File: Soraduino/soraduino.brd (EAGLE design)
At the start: 87.3 x 81.3 mm, 23 parts, among them IC1 ATMEGA168-AU, IC2 317EMP, IC3 317EMP

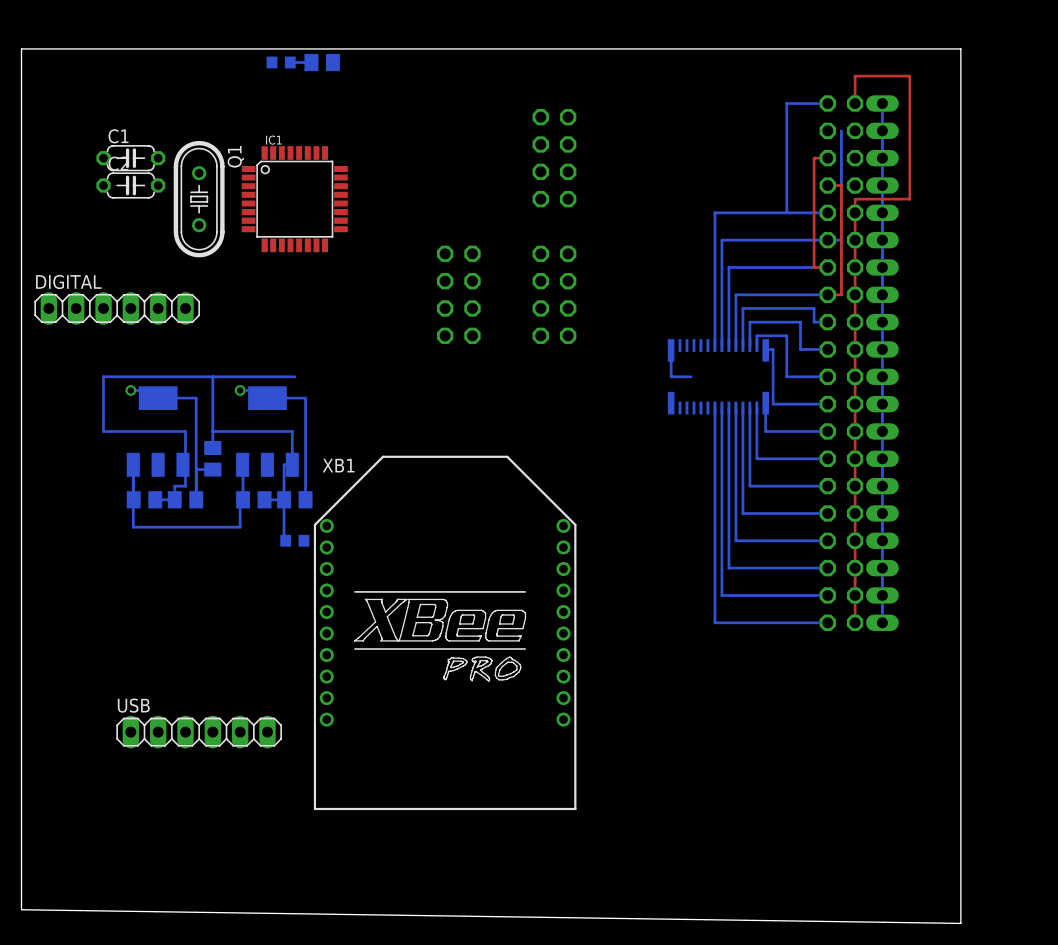
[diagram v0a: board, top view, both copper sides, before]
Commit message: 回路をとりあえず完成
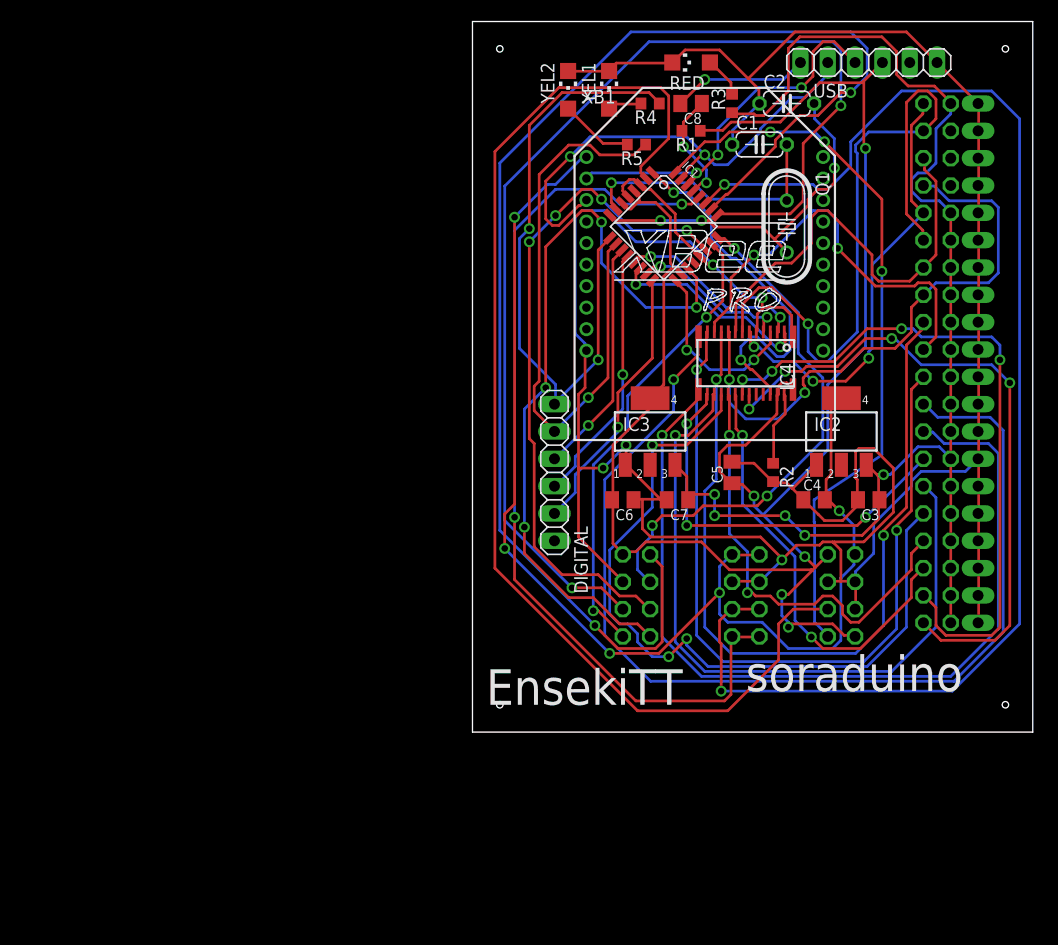
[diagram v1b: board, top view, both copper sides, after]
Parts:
- added R3, R4, R5: 1k, rcl:R0603
- added RED, YEL1, YEL2: (no value), led:CHIPLED_1206
- moved USB 88.0 mm to (91.4, 81.3)
- moved C2 61.4 mm to (83.8, 77.5)
- moved C1 58.4 mm to (81.3, 73.7)
- moved C3 57.1 mm to (91.4, 40.6), flipped to the top
- moved Q1 54.7 mm to (83.8, 66.0)
- moved IC2 53.3 mm to (88.9, 47.0), flipped to the top
- moved C7 49.5 mm to (73.7, 40.6), flipped to the top
- moved C5 48.3 mm to (78.7, 43.2), flipped to the top
- moved C4 48.3 mm to (86.4, 40.6), flipped to the top, turned to 0 degrees
- moved IC3 45.7 mm to (71.1, 47.0), flipped to the top
- moved GPS-SUP 45.2 mm to (88.9, 31.8)
- moved R2 44.9 mm to (82.5, 43.2), flipped to the top, turned to 270 degrees
- moved DIGITAL 43.4 mm to (62.2, 43.2), turned to 270 degrees
- moved XB1 41.9 mm to (76.2, 63.5)
- moved JAIRO-ANA 41.3 mm to (69.8, 31.8)
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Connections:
- new net N$10: R3.2, RED.A
- new net N$46: R4.2, YEL1.A
- new net N$48: R5.2, YEL2.A
- net GND: now also RED.C, YEL1.C, YEL2.C
- net N$39: now also R4.1
- net N$40: now also R5.1
- net VCC: now also R3.1
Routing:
- net GND: track 127.7 -> 290.3 mm, vias 0 -> 5
- net N$7: track 17.3 -> 167.5 mm, vias 0 -> 5
- net N$43: track 0.00 -> 125.0 mm, vias 0 -> 2
- net N$32: track 0.00 -> 124.3 mm, vias 0 -> 2
- net N$37: track 0.00 -> 108.9 mm
- net N$25: track 0.00 -> 106.6 mm, vias 0 -> 2
- net N$6: track 13.0 -> 113.3 mm, vias 0 -> 5
- net N$16: track 10.9 -> 99.2 mm, vias 0 -> 1
- net N$31: track 0.00 -> 85.1 mm, vias 0 -> 2
- net N$17: track 8.39 -> 83.1 mm, vias 0 -> 1
- net N$44: track 0.00 -> 69.6 mm, vias 0 -> 4
- net N$36: track 0.00 -> 68.0 mm, vias 0 -> 3
- net N$13: track 12.6 -> 76.5 mm, vias 0 -> 2
- net N$15: track 11.3 -> 74.0 mm, vias 0 -> 2
- net N$45: track 0.00 -> 62.5 mm, vias 0 -> 4
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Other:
- board size 87.3 x 81.3 mm -> 52.1 x 66 mm
- board text added: "EnsekiTT"
- board text added: "soraduino"
